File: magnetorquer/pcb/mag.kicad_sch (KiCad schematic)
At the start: 0 parts

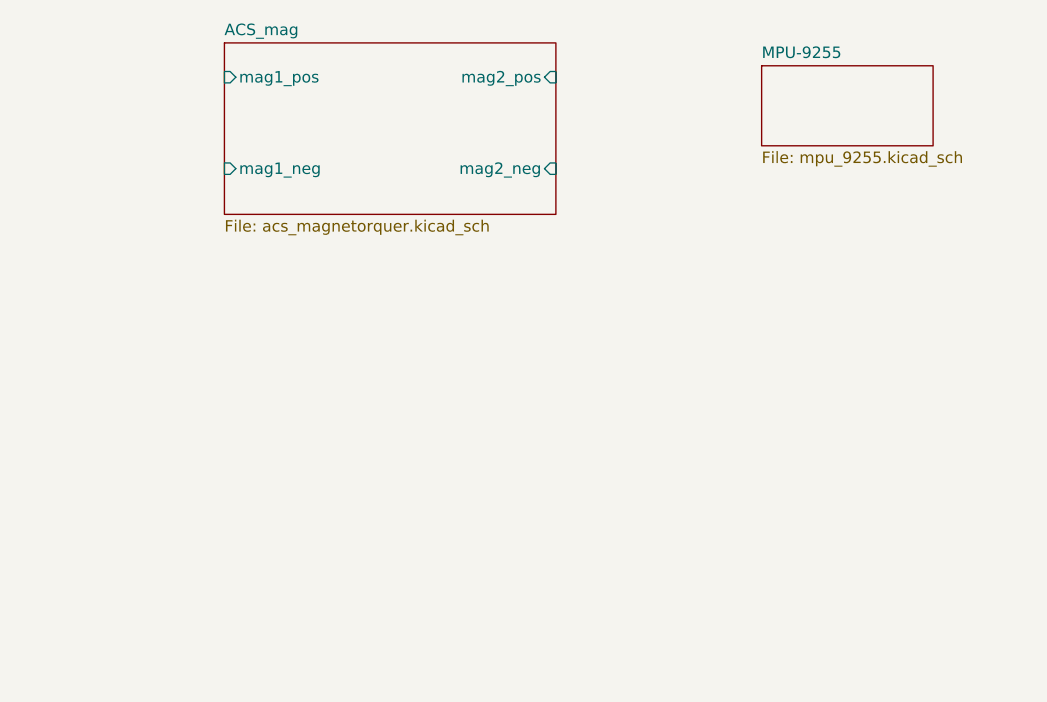
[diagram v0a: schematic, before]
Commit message: Alt det der manglede til Kicad
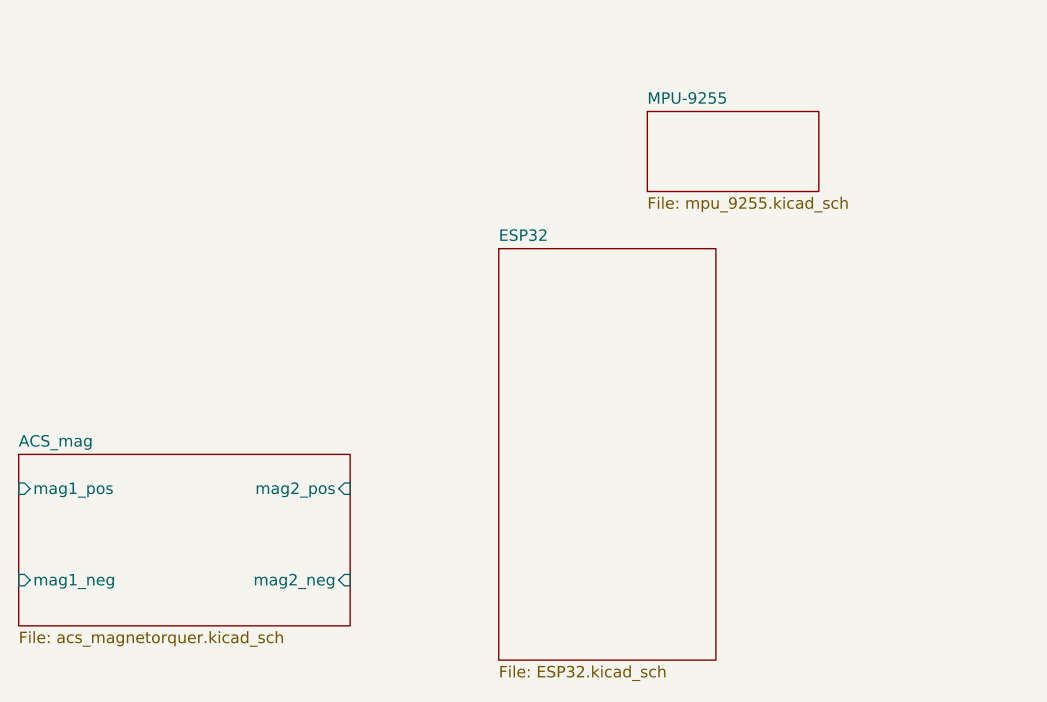
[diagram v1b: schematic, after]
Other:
- added sheet ESP32 (ESP32.kicad_sch)
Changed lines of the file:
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@@
 	(paper "A4")
 	(sheet
-		(at 58.42 55.88)
+		(at 35.56 101.6)
 		(size 36.83 19.05)
 		(exclude_from_sim no)
@@
 		)
 		(property "Sheetname" "ACS_mag"
-			(at 58.42 55.1684 0)
+			(at 35.56 100.8884 0)
 			(effects
 				(font
@@
 		)
 		(property "Sheetfile" "acs_magnetorquer.kicad_sch"
-			(at 58.42 75.5146 0)
+			(at 35.56 121.2346 0)
 			(effects
 				(font
@@
 		)
 		(pin "mag1_neg" input
-			(at 58.42 69.85 180)
+			(at 35.56 115.57 180)
 			(effects
 				(font
@@
 		)
 		(pin "mag1_pos" input
-			(at 58.42 59.69 180)
+			(at 35.56 105.41 180)
 			(effects
 				(font
@@
 		)
 		(pin "mag2_neg" input
-			(at 95.25 69.85 0)
+			(at 72.39 115.57 0)
 			(effects
 				(font
@@
 		)
 		(pin "mag2_pos" input
-			(at 95.25 59.69 0)
+			(at 72.39 105.41 0)
 			(effects
 				(font
@@
 	)
 	(sheet
-		(at 118.11 58.42)
+		(at 88.9 78.74)
+		(size 24.13 45.72)
+		(exclude_from_sim no)
+		(in_bom yes)
+		(on_board yes)
+		(dnp no)
+		(fields_autoplaced yes)
+		(stroke
+			(width 0.1524)
+			(type solid)
+		)
+		(fill
+			(color 0 0 0 0.0000)
+		)
+		(property "Sheetname" "ESP32"
+			(at 88.9 78.0284 0)
+			(effects
+				(font
+					(size 1.27 1.27)
+				)
+				(justify left bottom)
+			)
+		)
+		(property "Sheetfile" "ESP32.kicad_sch"
+			(at 88.9 125.0446 0)
+			(effects
+				(font
+					(size 1.27 1.27)
+				)
+				(justify left top)
+			)
+		)
+		(instances
+			(project "mag"
+				(path "/14c04de7-71ee-4f20-9e6e-041dbb035733"
+					(page "4")
+				)
+			)
+		)
+	)
+	(sheet
+		(at 105.41 63.5)
 		(size 19.05 8.89)
 		(exclude_from_sim no)
@@
 		)
 		(property "Sheetname" "MPU-9255"
-			(at 118.11 57.7084 0)
+			(at 105.41 62.7884 0)
 			(effects
 				(font
@@
 		)
 		(property "Sheetfile" "mpu_9255.kicad_sch"
-			(at 118.11 67.8946 0)
+			(at 105.41 72.9746 0)
 			(effects
 				(font
